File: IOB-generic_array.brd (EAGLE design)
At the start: 104.1 x 106.7 mm, 33 parts

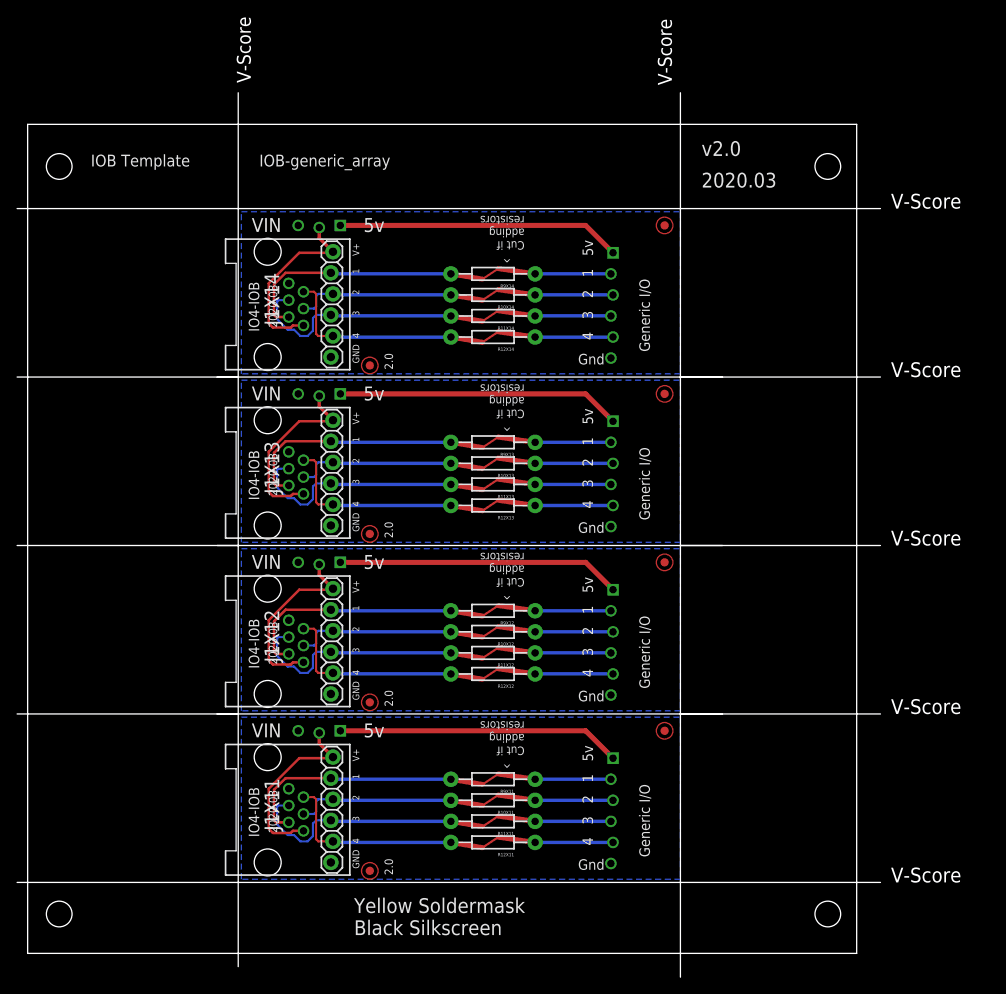
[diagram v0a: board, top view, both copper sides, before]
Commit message: silkscreen and top fill, array
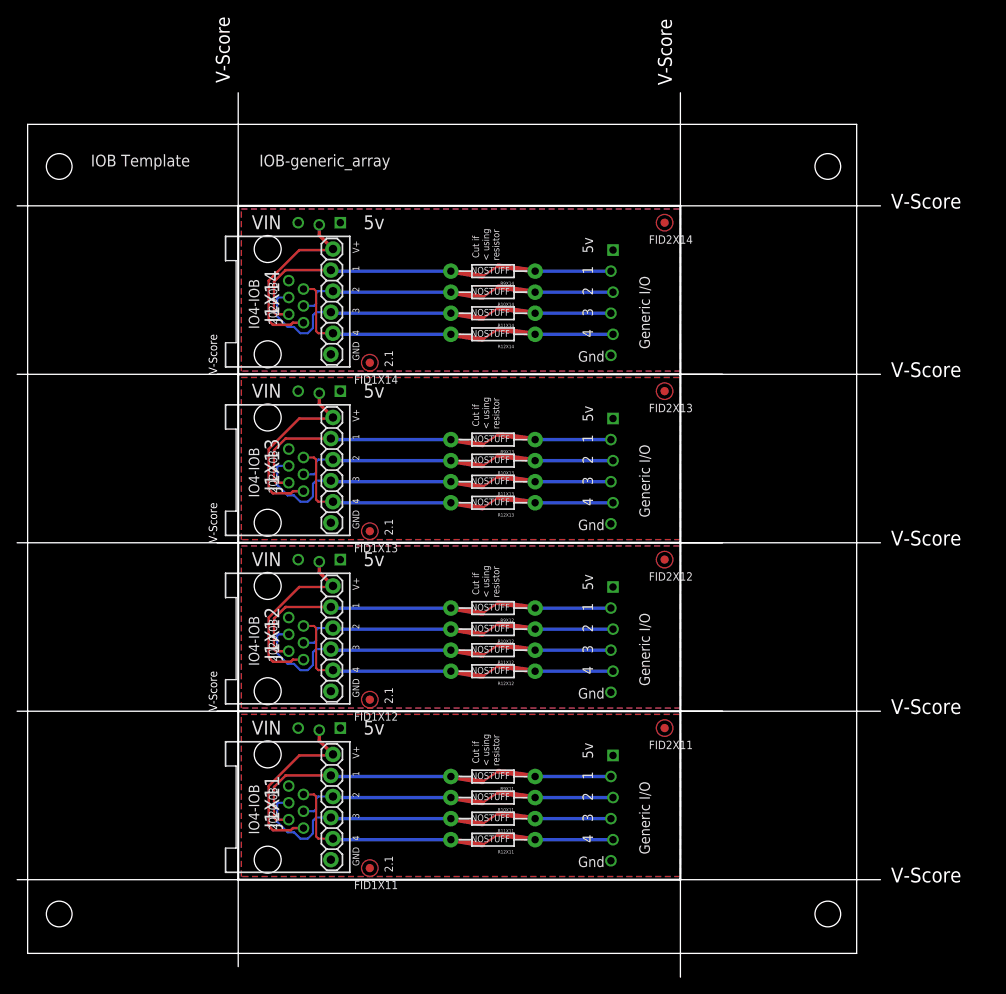
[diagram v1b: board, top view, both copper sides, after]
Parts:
- FID1X11, FID1X12, FID1X13, FID1X14, FID2X11, FID2X12, FID2X13, FID2X14: value (none) -> FIDUCIAL
- IOBX11, IOBX12, IOBX13, IOBX14: value (none) -> CONNECTOR-IO4-IOBFULL
- J1X11, J1X12, J1X13, J1X14: value (none) -> RJ12/6
- R10X11, R10X12, R10X13, R10X14, R11X11, R11X12, R11X13, R11X14, R12X11, R12X12, R12X13, R12X14, R9X11, R9X12, R9X13, R9X14: value (none) -> NOSTUFF
- moved R9X14 0.33 mm to (56.1, 82.3)
- moved FID2X11 0.33 mm to (76.8, 27.2)
- moved IOBX12 0.33 mm to (25.4, 29.2)
- moved FID1X11 0.33 mm to (41.3, 10.3)
- moved IOBX11 0.33 mm to (25.4, 8.89)
- moved R11X11 0.33 mm to (56.1, 16.3)
- moved R12X11 0.33 mm to (56.1, 13.7)
- moved FID1X12 0.33 mm to (41.3, 30.6)
- moved FID1X13 0.33 mm to (41.3, 50.9)
- moved FID1X14 0.33 mm to (41.3, 71.2)
- moved FID2X12 0.33 mm to (76.8, 47.5)
- moved FID2X13 0.33 mm to (76.8, 67.8)
- moved FID2X14 0.33 mm to (76.8, 88.1)
- moved IOBX13 0.33 mm to (25.4, 49.5)
- moved IOBX14 0.33 mm to (25.4, 69.8)
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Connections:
- removed net VCCX11: IOBX11.V5, IOBX11.V5@1
- removed net VCCX12: IOBX12.V5, IOBX12.V5@1
- removed net VCCX13: IOBX13.V5, IOBX13.V5@1
- removed net VCCX14: IOBX14.V5, IOBX14.V5@1
- new net VINX11: IOBX11.V+
- new net VINX12: IOBX12.V+
- new net VINX13: IOBX13.V+
- new net VINX14: IOBX14.V+
- net VCCIOX11: now also IOBX11.V5, IOBX11.V5@1; no longer IOBX11.V+
- net VCCIOX12: now also IOBX12.V5, IOBX12.V5@1; no longer IOBX12.V+
- net VCCIOX13: now also IOBX13.V5, IOBX13.V5@1; no longer IOBX13.V+
- net VCCIOX14: now also IOBX14.V5, IOBX14.V5@1; no longer IOBX14.V+
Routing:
- net VCCX14: track 34.3 -> 0.00 mm
- net VCCX13: track 34.3 -> 0.00 mm
- net VCCX12: track 34.3 -> 0.00 mm
- net VCCX11: track 34.3 -> 0.00 mm
- added copper zone on layer 1, net VCCIOX11
- added copper zone on layer 1, net VCCIOX12
- added copper zone on layer 1, net VCCIOX13
- added copper zone on layer 1, net VCCIOX14
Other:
- outline, holes or cut-outs redrawn
- board text added: "2.1"
- board text added: "Cut if < using resistor"
- board text added: "FID1"
- board text added: "FID2"
- board text added: "R10"
- board text added: "R11"
- board text added: "R12"
- board text added: "R9"
- board text added: "V-Score"
- board text added: "Yellow Headers"
- board text added: "Yellow Soldermask White Silkscreen"
- board text removed: "2.0"
- board text removed: "Yellow Soldermask Black Silkscreen"
- board text removed: "^ Cut if adding resistors"
- board text removed: "v2.0"
